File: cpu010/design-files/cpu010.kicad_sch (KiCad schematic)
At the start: 0 parts

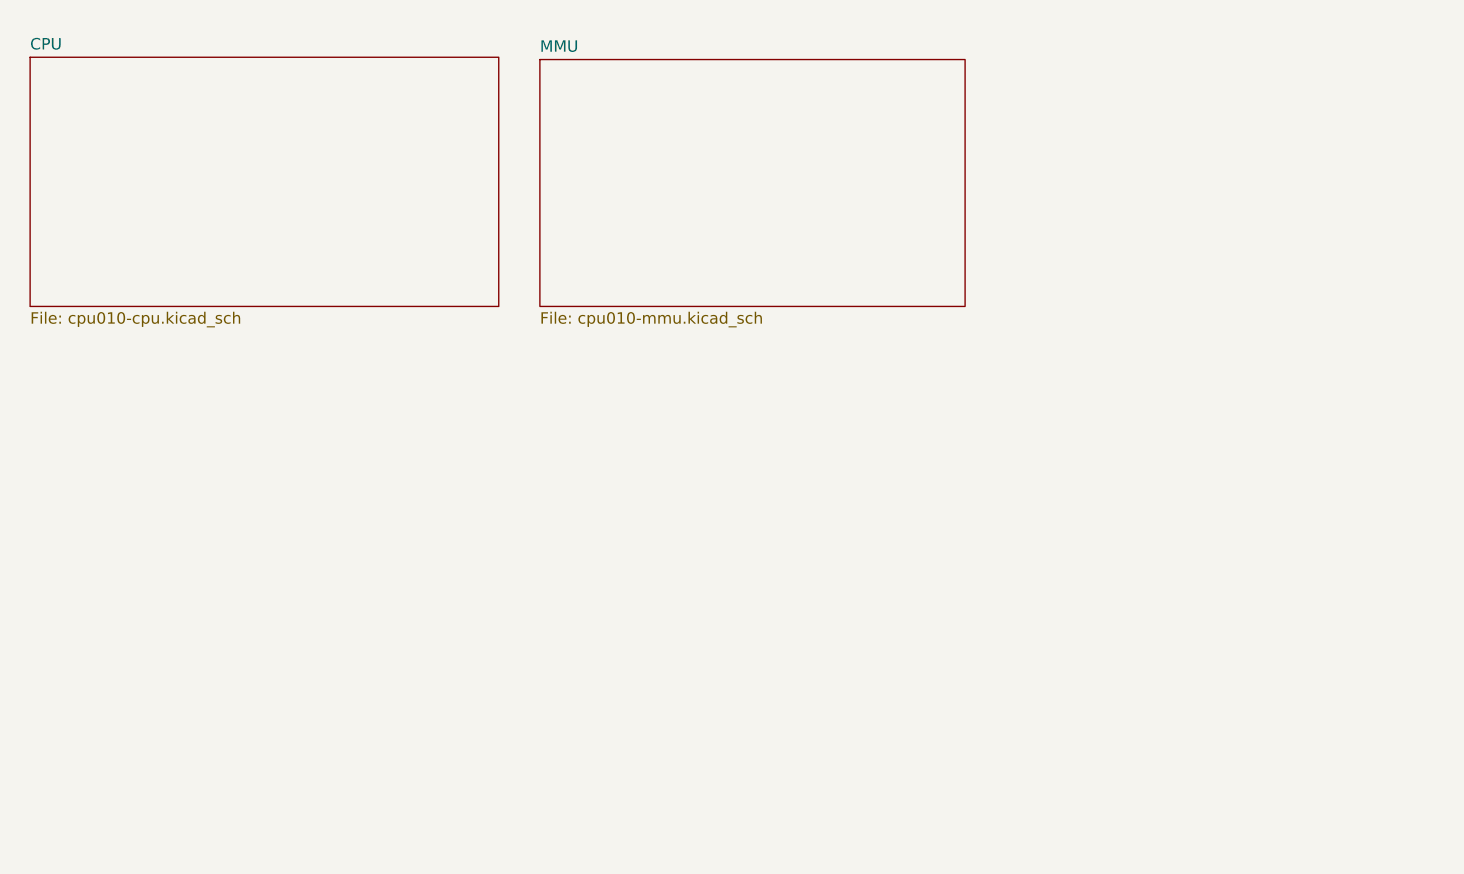
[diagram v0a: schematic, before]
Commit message: Add a bunch of Control Space stuff.
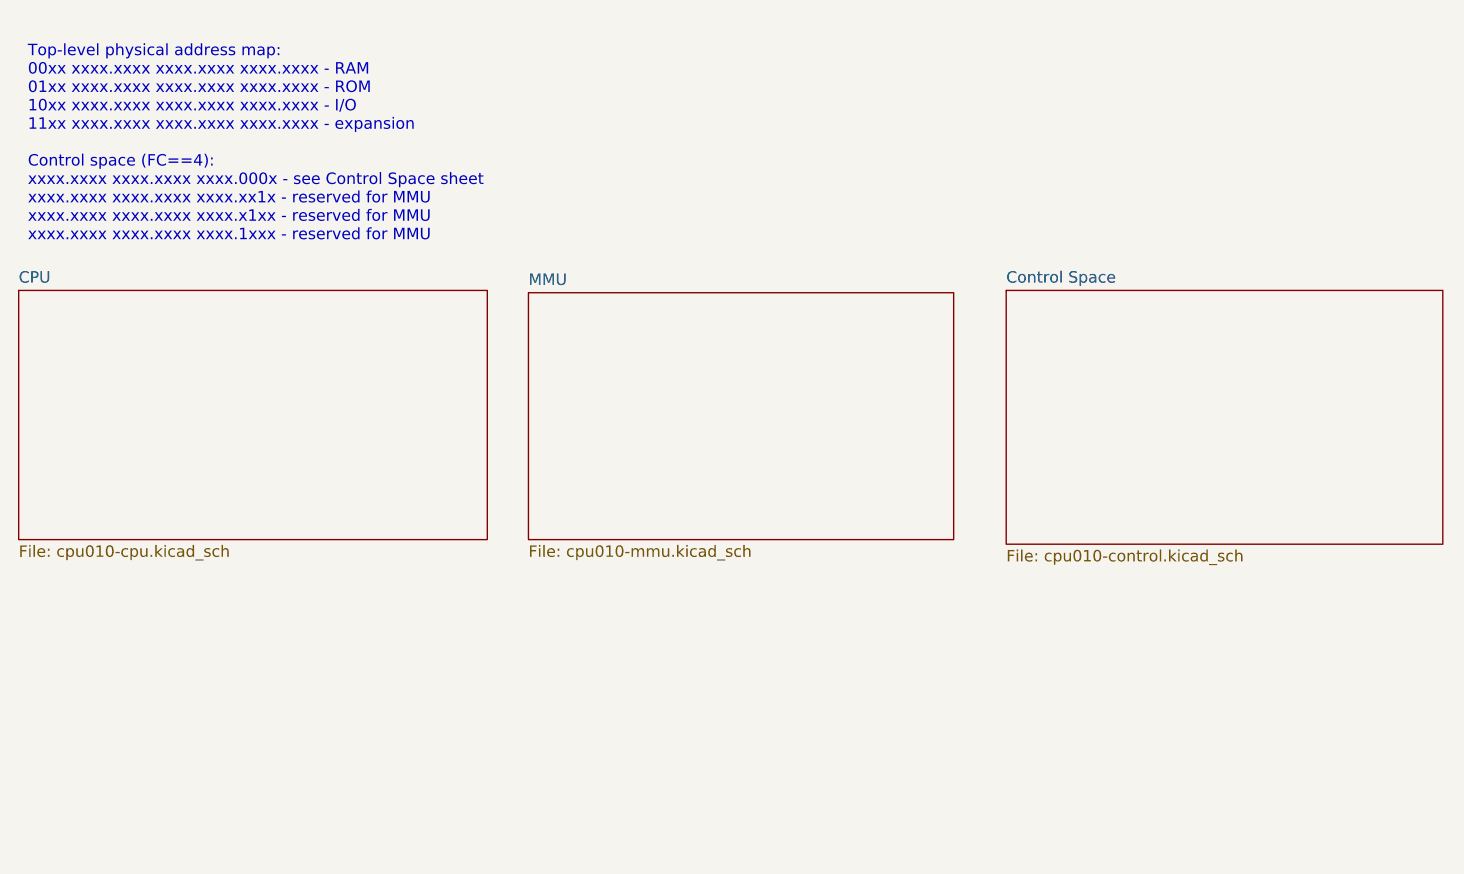
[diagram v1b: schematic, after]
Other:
- added sheet Control Space (cpu010-control.kicad_sch)
- note added: "Top-level physical address map: 00xx xxxx.xxxx xxxx.xxxx xxxx.xxxx - RAM 01xx xxxx.xxxx xxxx.xxxx xxxx.xxxx - ROM 10xx xxxx.xxxx xxxx.xxxx xxxx.xxxx - I/O 11xx xxxx.xxxx xxxx.xxxx xxxx.xxxx - expansion Control space (FC==4): xxxx.xxxx xxxx.xxxx xxxx.000x - see Control Space sheet xxxx.xxxx xxxx.xxxx xxxx.xx1x - reserved for MMU xxxx.xxxx xxxx.xxxx xxxx.x1xx - reserved for MMU xxxx.xxxx xxxx.xxxx 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"
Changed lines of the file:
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@@
 	(generator_version "9.0")
 	(paper "A4")
+	(text "Top-level physical address map:\n00xx xxxx.xxxx xxxx.xxxx xxxx.xxxx - RAM\n01xx xxxx.xxxx xxxx.xxxx xxxx.xxxx - ROM\n10xx xxxx.xxxx xxxx.xxxx xxxx.xxxx - I/O\n11xx xxxx.xxxx xxxx.xxxx xxxx.xxxx - expansion\n\nControl space (FC==4):\nxxxx.xxxx xxxx.xxxx xxxx.000x - see Control Space sheet\nxxxx.xxxx xxxx.xxxx xxxx.xx1x - reserved for MMU\nxxxx.xxxx xxxx.xxxx xxxx.x1xx - reserved for MMU\nxxxx.xxxx xxxx.xxxx xxxx.1xxx - reserved for MMU"
+		(exclude_from_sim no)
+		(at 18.034 29.21 0)
+		(effects
+			(font
+				(size 1.27 1.27)
+			)
+			(justify left)
+		)
+	)
 	(sheet
-		(at 18.288 19.558)
+		(at 17.018 45.466)
 		(size 52.07 27.686)
 		(exclude_from_sim no)
@@
 		)
 		(property "Sheetname" "CPU"
-			(at 18.288 18.8464 0)
+			(at 17.018 44.7544 0)
 			(effects
 				(font
@@
 		)
 		(property "Sheetfile" "cpu010-cpu.kicad_sch"
-			(at 18.288 47.8286 0)
+			(at 17.018 73.7366 0)
 			(effects
 				(font
@@
 	)
 	(sheet
-		(at 74.93 19.812)
+		(at 126.746 45.466)
+		(size 48.514 28.194)
+		(exclude_from_sim no)
+		(in_bom yes)
+		(on_board yes)
+		(dnp no)
+		(fields_autoplaced yes)
+		(stroke
+			(width 0.1524)
+			(type solid)
+		)
+		(fill
+			(color 0 0 0 0.0000)
+		)
+		(property "Sheetname" "Control Space"
+			(at 126.746 44.7544 0)
+			(effects
+				(font
+					(size 1.27 1.27)
+				)
+				(justify left bottom)
+			)
+		)
+		(property "Sheetfile" "cpu010-control.kicad_sch"
+			(at 126.746 74.2446 0)
+			(effects
+				(font
+					(size 1.27 1.27)
+				)
+				(justify left top)
+			)
+		)
+		(instances
+			(project "cpu010"
+				(path "/65f80d66-eea1-4882-b29a-ae1b65892b55"
+					(page "4")
+				)
+			)
+		)
+	)
+	(sheet
+		(at 73.66 45.72)
 		(size 47.244 27.432)
 		(exclude_from_sim no)
@@
 		)
 		(property "Sheetname" "MMU"
-			(at 74.93 19.1004 0)
+			(at 73.66 45.0084 0)
 			(effects
 				(font
@@
 		)
 		(property "Sheetfile" "cpu010-mmu.kicad_sch"
-			(at 74.93 47.8286 0)
+			(at 73.66 73.7366 0)
 			(effects
 				(font

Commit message: Fix up the Enable register.
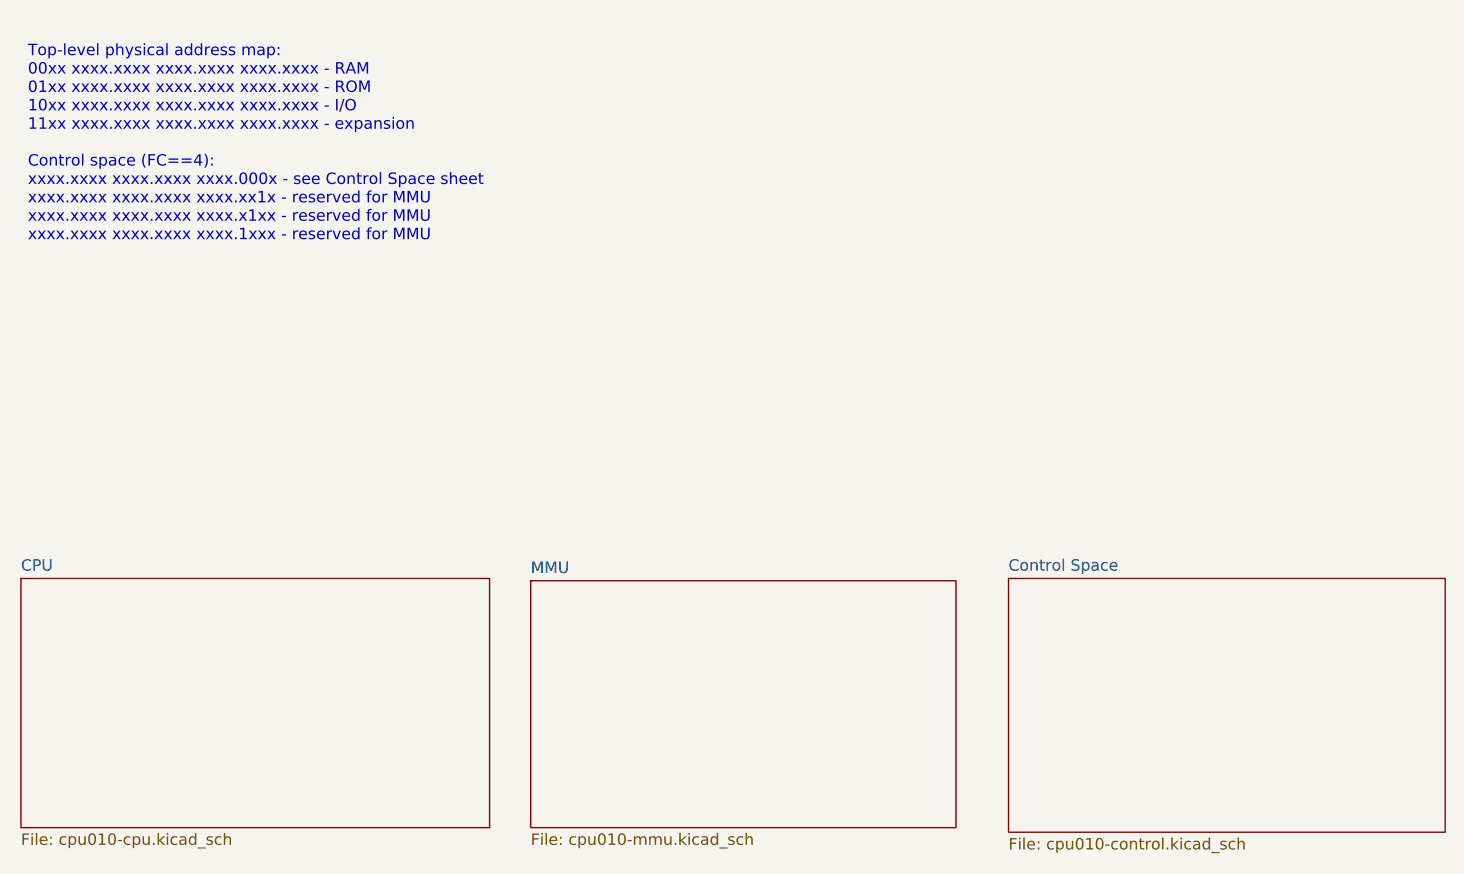
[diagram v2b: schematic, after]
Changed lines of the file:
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@@
 	)
 	(sheet
-		(at 17.018 45.466)
+		(at 17.272 77.47)
 		(size 52.07 27.686)
 		(exclude_from_sim no)
@@
 		)
 		(property "Sheetname" "CPU"
-			(at 17.018 44.7544 0)
+			(at 17.272 76.7584 0)
 			(effects
 				(font
@@
 		)
 		(property "Sheetfile" "cpu010-cpu.kicad_sch"
-			(at 17.018 73.7366 0)
+			(at 17.272 105.7406 0)
 			(effects
 				(font
@@
 	)
 	(sheet
-		(at 126.746 45.466)
+		(at 127 77.47)
 		(size 48.514 28.194)
 		(exclude_from_sim no)
@@
 		)
 		(property "Sheetname" "Control Space"
-			(at 126.746 44.7544 0)
+			(at 127 76.7584 0)
 			(effects
 				(font
@@
 		)
 		(property "Sheetfile" "cpu010-control.kicad_sch"
-			(at 126.746 74.2446 0)
+			(at 127 106.2486 0)
 			(effects
 				(font
@@
 	)
 	(sheet
-		(at 73.66 45.72)
+		(at 73.914 77.724)
 		(size 47.244 27.432)
 		(exclude_from_sim no)
@@
 		)
 		(property "Sheetname" "MMU"
-			(at 73.66 45.0084 0)
+			(at 73.914 77.0124 0)
 			(effects
 				(font
@@
 		)
 		(property "Sheetfile" "cpu010-mmu.kicad_sch"
-			(at 73.66 73.7366 0)
+			(at 73.914 105.7406 0)
 			(effects
 				(font

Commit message: Add top-level address decoding.
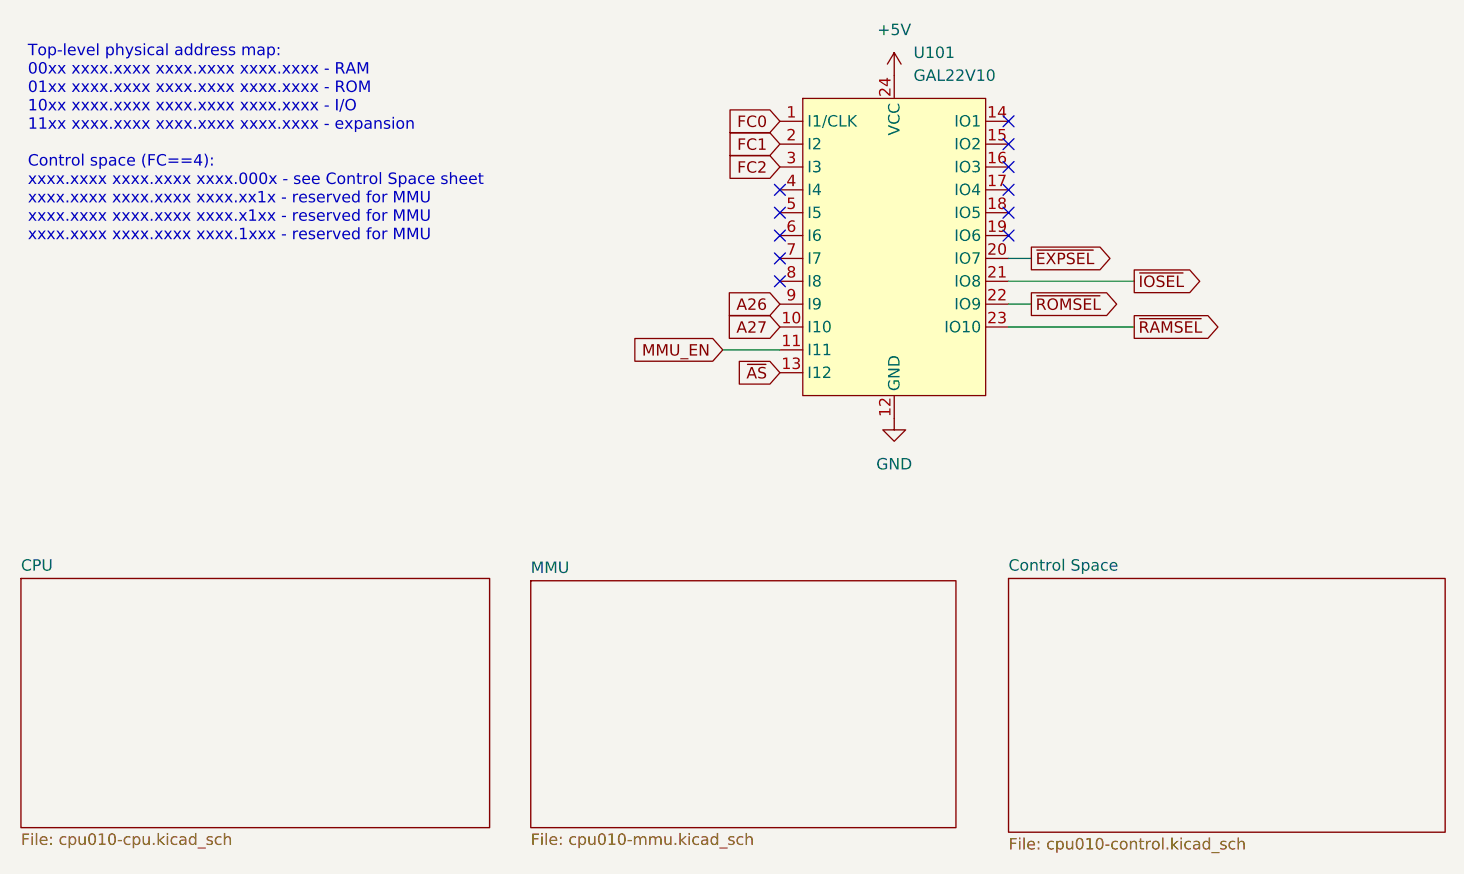
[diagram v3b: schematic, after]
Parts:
- added U101: GAL22V10, Package_DIP:DIP-24_W7.62mm_Socket, symbol jrt-ICs:GAL22V10
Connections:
- new net +5V: U101.24 (VCC)
- new net A26: U101.9 (I9)
- new net A27: U101.10 (I10)
- new net FC0: U101.1 (I1/CLK)
- new net FC1: U101.2 (I2)
- new net FC2: U101.3 (I3)
- new net GND: U101.12 (GND)
- new net MMU_EN: U101.11 (I11)
- new net ~{AS}: U101.13 (I12)
- new net ~{EXPSEL}: U101.20 (IO7)
- new net ~{IOSEL}: U101.21 (IO8)
- new net ~{RAMSEL}: U101.23 (IO10)
- new net ~{ROMSEL}: U101.22 (IO9)
- no-connect marks 0 -> 11
